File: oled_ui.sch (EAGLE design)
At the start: 25 parts, among them IC1 74HC14D

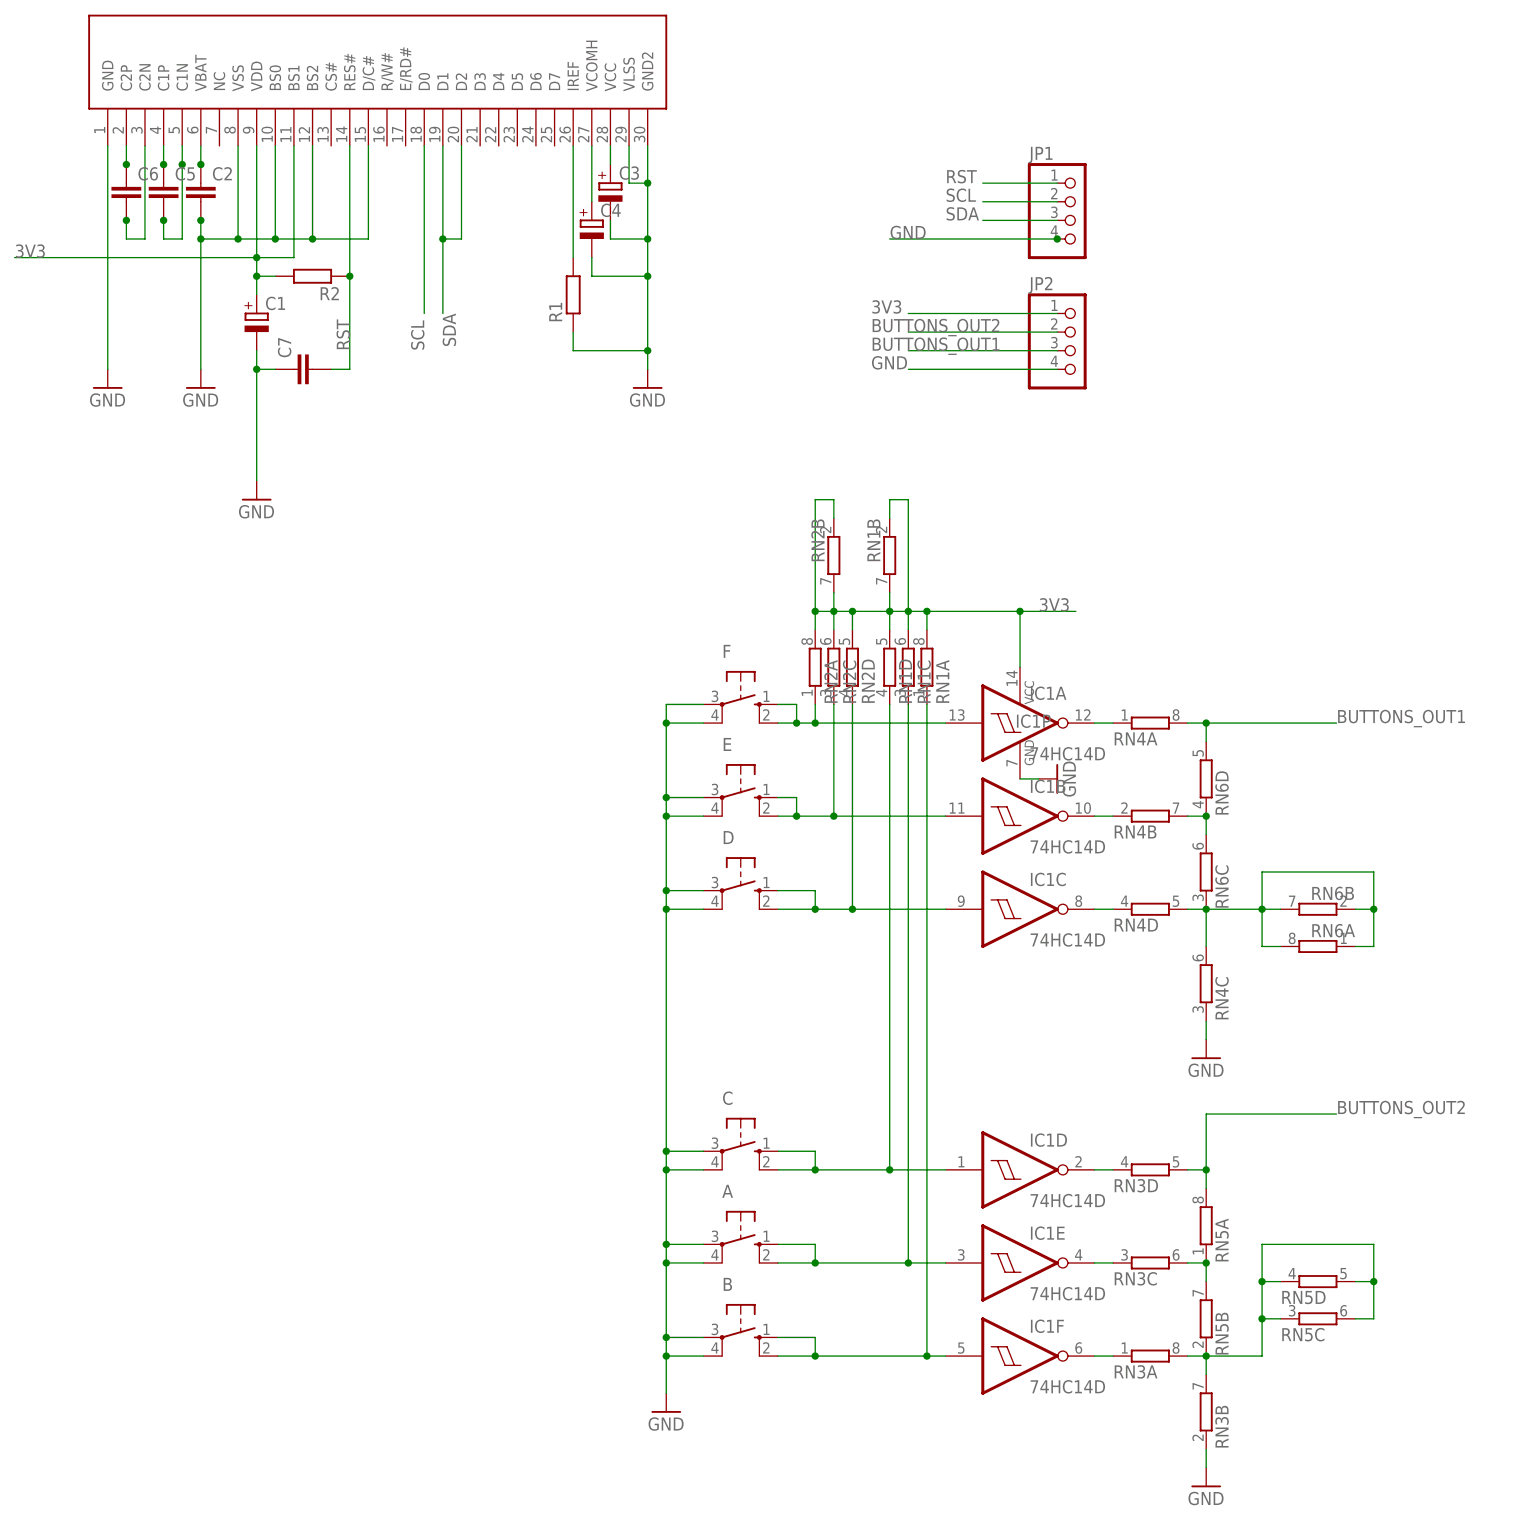
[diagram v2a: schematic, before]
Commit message: work in progress
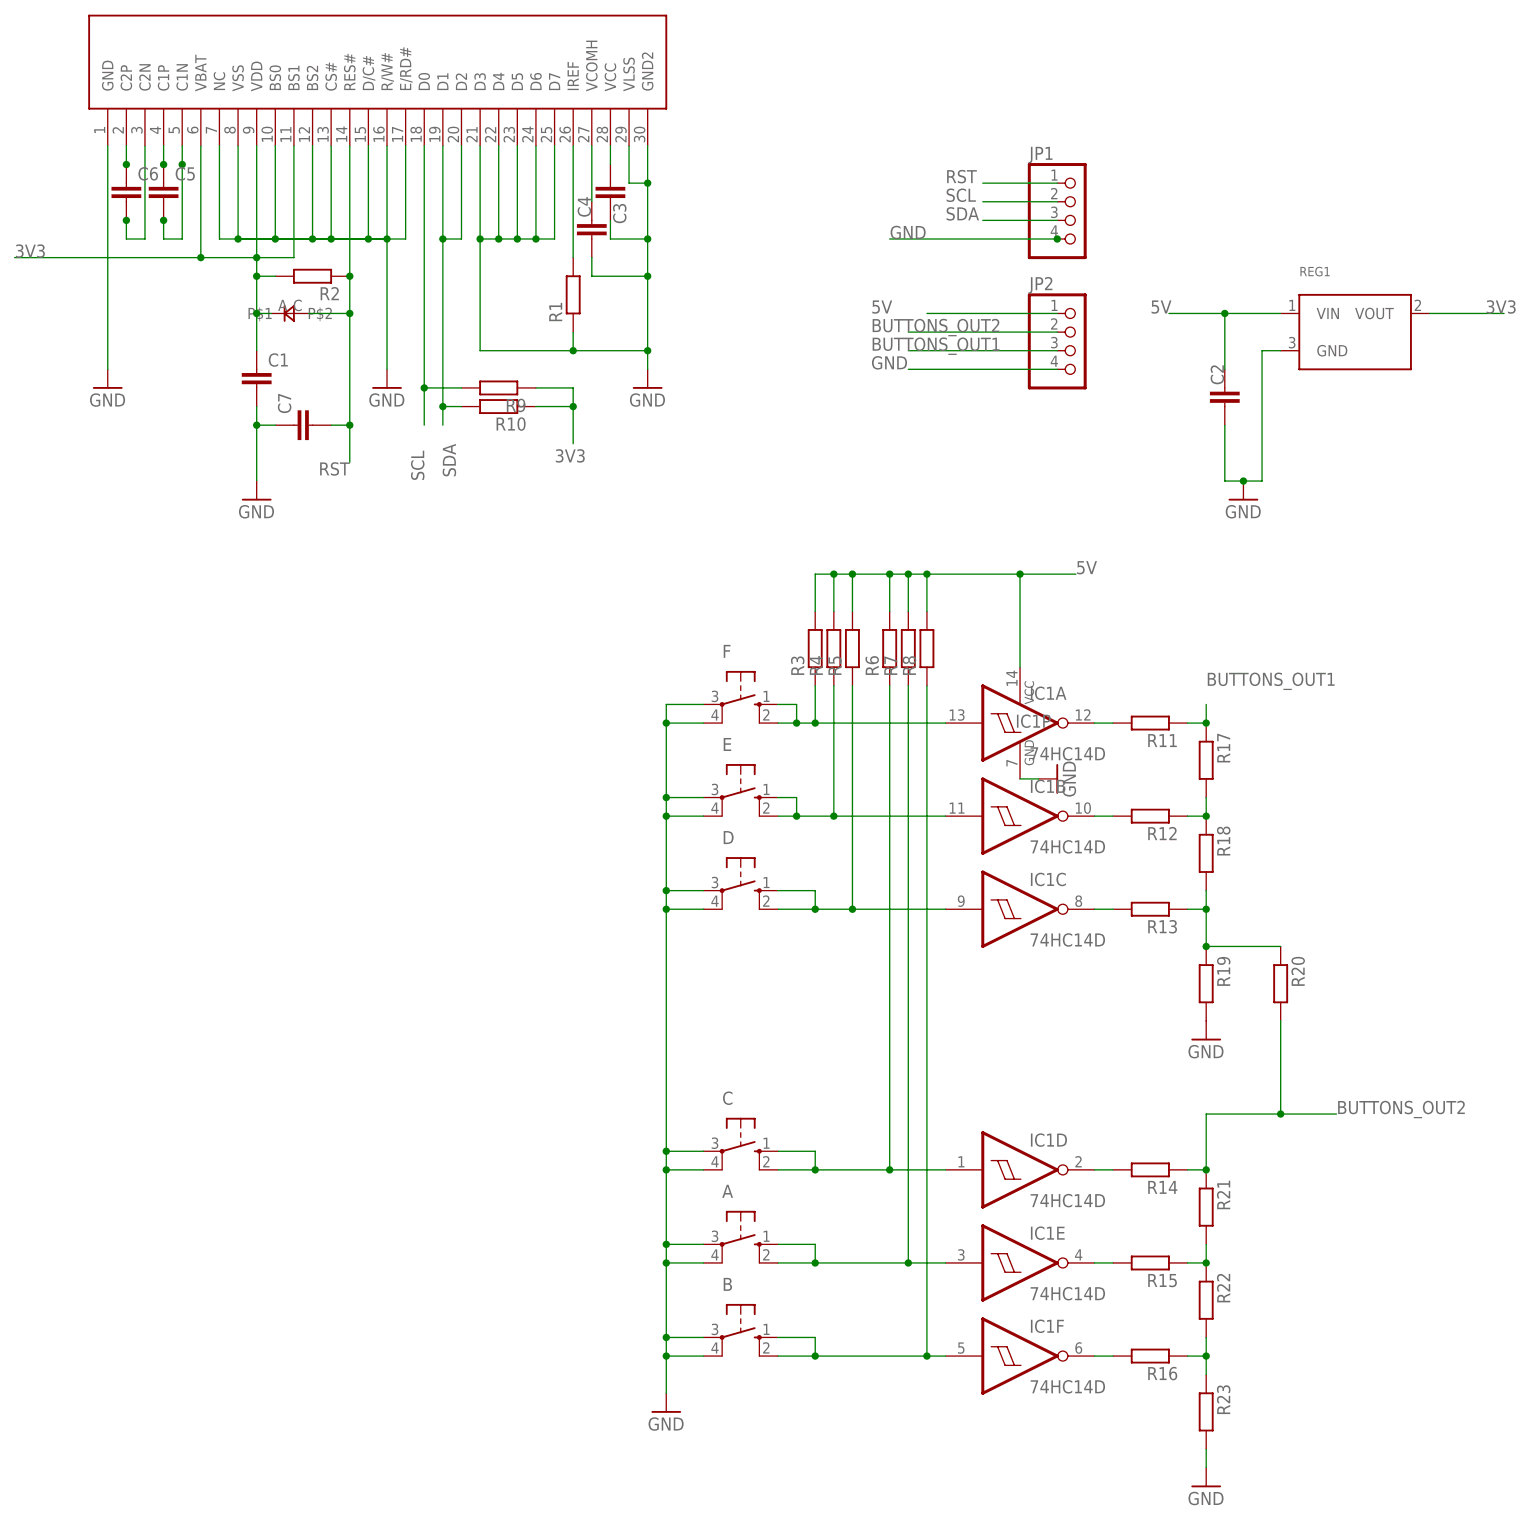
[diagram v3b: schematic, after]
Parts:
- removed RN1, RN2, RN3, RN4, RN5, RN6: (no value), resistor-dil:4R-NCAY16
- added D1: 0805DIODE, jasons_stuff:0805DIODE
- added R10, R11, R12, R13, R14, R15, R16, R17, R18, R19, R20, R21, R22, R23, R3, R4, R5, R6, R7, R8, R9: (no value), rcl:R-EU_R0805
- added REG1: (no value), microbuilder:VREG_SOT23
- C1, C3: device resistor:CPOL-EUSMCA -> rcl:C-EUC0805
- C4: device resistor:CPOL-EUSMCB -> rcl:C-EUC0805
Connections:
- removed net N$19: IC1D.O, RN3D.1
- removed net N$26: RN3A.2, RN3B.2, RN5B.1, RN5C.1, RN5C.2, RN5D.1, RN5D.2
- new net 5V: C2.1, IC1P.VCC, JP2.1, R3.2, R4.2, R5.2, R6.2, R7.2, R8.2, REG1.VIN
- new net N$24: IC1A.O, R11.2
- net 3V3: now also C1.1, D1.P$2, R10.1, R9.1, REG1.VOUT, U$1.VBAT; no longer C1.+, IC1P.VCC, JP2.1, RN1A.2, RN1B.1, RN1B.2, RN1C.2, RN1D.2, RN2A.2, RN2B.1, RN2B.2, RN2C.2, RN2D.2
- net BUTTONS_OUT1: now also R11.1, R17.1; no longer RN4A.2, RN6D.2
- net BUTTONS_OUT2: now also R14.1, R20.2, R21.1; no longer RN3D.2, RN5A.2
- net GND: now also C1.2, C3.2, C4.2, R19.2, R23.2, REG1.GND, U$1.CS#, U$1.D3, U$1.D4, U$1.D5, U$1.D6, U$1.D7, U$1.E/RD#, U$1.NC, U$1.R/W#; no longer C1.-, C3.-, C4.-, RN3B.1, RN4C.1
- net N$11: now also R6.1; no longer RN1D.1
- net N$12: now also R5.1; no longer RN2D.1
- net N$13: now also R4.1; no longer RN2C.1
- net N$14: now also R3.1; no longer RN2A.1
- net N$15: now also IC1E.O, R15.2; no longer IC1A.O, RN4A.1
- net N$16: now also IC1F.O, R16.2; no longer IC1B.O, RN4B.1
- net N$17: now also R16.1, R22.2, R23.1; no longer IC1C.O, RN4D.1
- net N$18: now also R15.1, R21.2, R22.1; no longer IC1E.O, RN3C.1
- net N$20: now also IC1C.O, R13.2; no longer IC1F.O, RN3A.1
- net N$21: now also R13.1, R18.2, R19.1, R20.1; no longer RN4B.2, RN6C.2, RN6D.1
- net N$22: now also IC1B.O, R12.2; no longer RN4C.2, RN4D.2, RN6A.1, RN6A.2, RN6B.1, RN6B.2, RN6C.1
- net N$23: now also R12.1, R17.2, R18.1; no longer RN3C.2, RN5A.1, RN5B.2
- net N$5: now also R8.1; no longer RN1A.1
- net N$6: now also C3.1; no longer C3.+
- net N$7: now also IC1D.O, R14.2; no longer C2.1, U$1.VBAT
- net N$8: now also C4.1; no longer C4.+
- net N$9: now also R7.1; no longer RN1C.1
- net RST: now also D1.P$1
- net SCL: now also R9.2
- net SDA: now also R10.2
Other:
- moved on the sheet: C2, C7
